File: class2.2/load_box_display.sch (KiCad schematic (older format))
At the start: 10 parts, among them P1 FPC-30

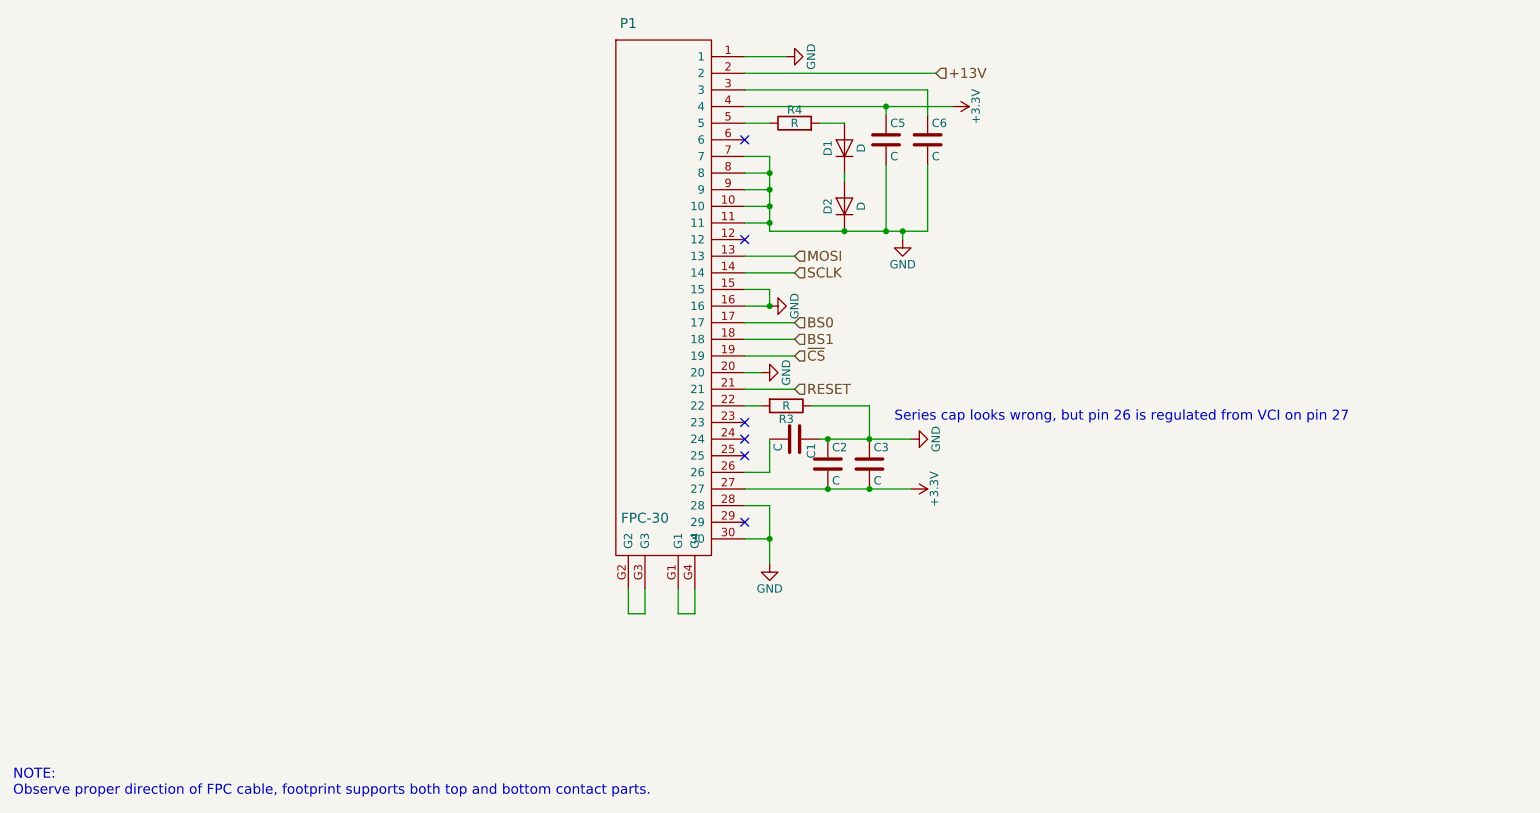
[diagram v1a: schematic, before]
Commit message: Checkpoint with NHD, 3.3v, and layout
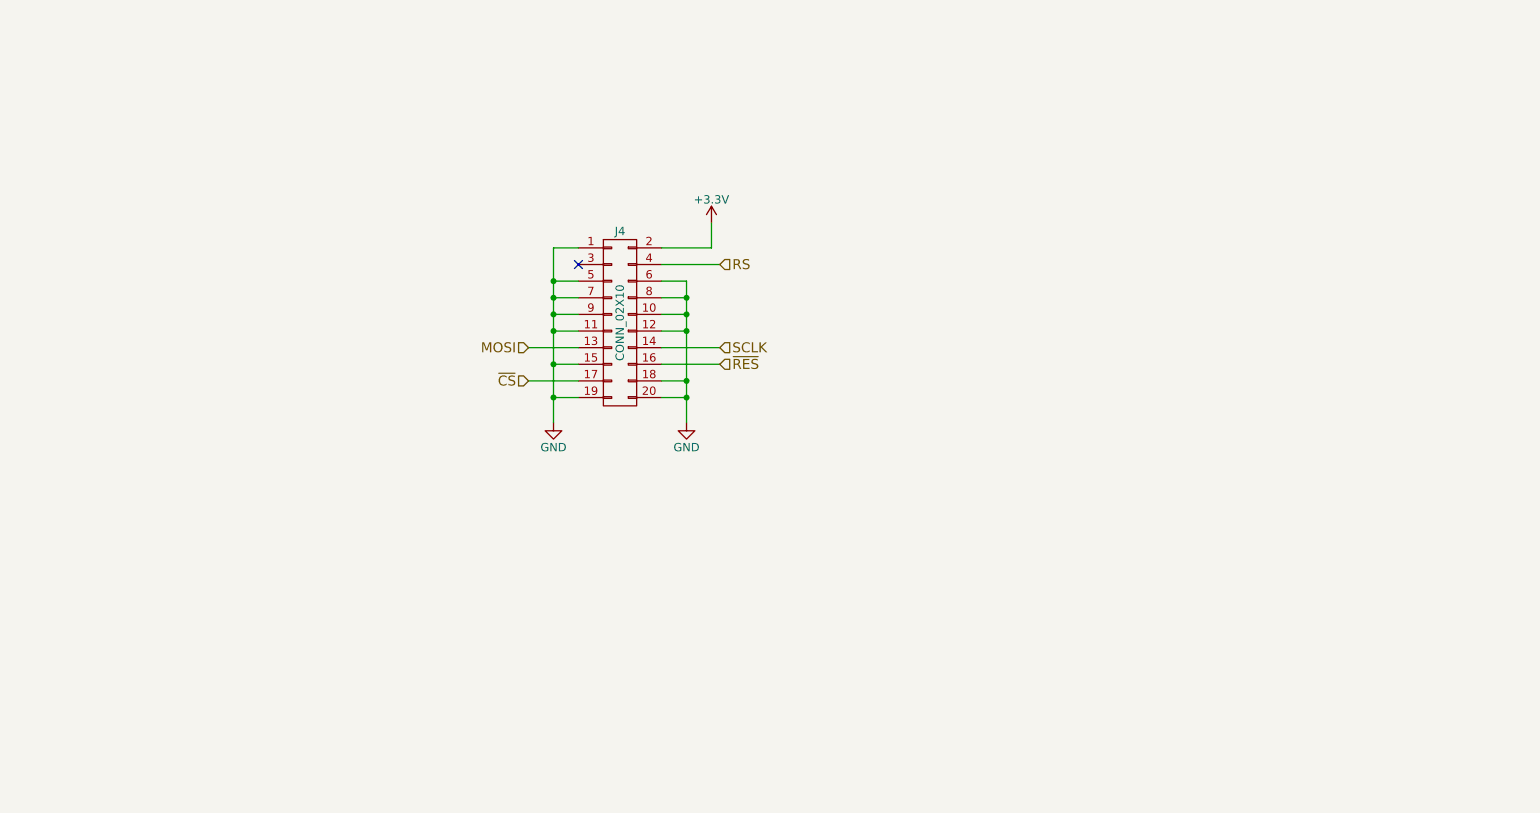
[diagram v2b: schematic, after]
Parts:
- removed C1, C2, C3, C5, C6: C, Capacitors_SMD:C_0603, symbol C
- removed D1, D2: D, Diodes_SMD:D_SOD-123, symbol D
- removed P1: FPC-30, symbol FPC-30
- removed R3, R4: R, Resistors_SMD:R_0603, symbol R
- added J4: CONN_02X10, nhd:NHD-1.69, symbol CONN_02X10
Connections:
- net +3V3: now also J4.2 (P2)
- net GND: now also J4.1 (P1), J4.10 (P10), J4.11 (P11), J4.12 (P12), J4.15 (P15), J4.18 (P18), J4.19 (P19), J4.20 (P20), J4.5 (P5), J4.6 (P6), J4.7 (P7), J4.8 (P8), J4.9 (P9)
- net MOSI: now also J4.13 (P13)
- net SCLK: now also J4.14 (P14)
- net ~CS: now also J4.17 (P17)
- new net RS: J4.4 (P4)
- new net ~RES: J4.16 (P16)
- no-connect marks 6 -> 1
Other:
- note removed: "NOTE:\nObserve proper direction of FPC cable, footprint supports both top and bottom contact parts."
- note removed: "Series cap looks wrong, but pin 26 is regulated from VCI on pin 27"
